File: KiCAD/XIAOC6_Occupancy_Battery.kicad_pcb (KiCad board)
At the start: 4 copper layers, 43.5 x 29.5 mm, 6 parts, among them U1 ZC362800_, U2 XIAO-ESP32-S3-SMD, U3 SHTC3

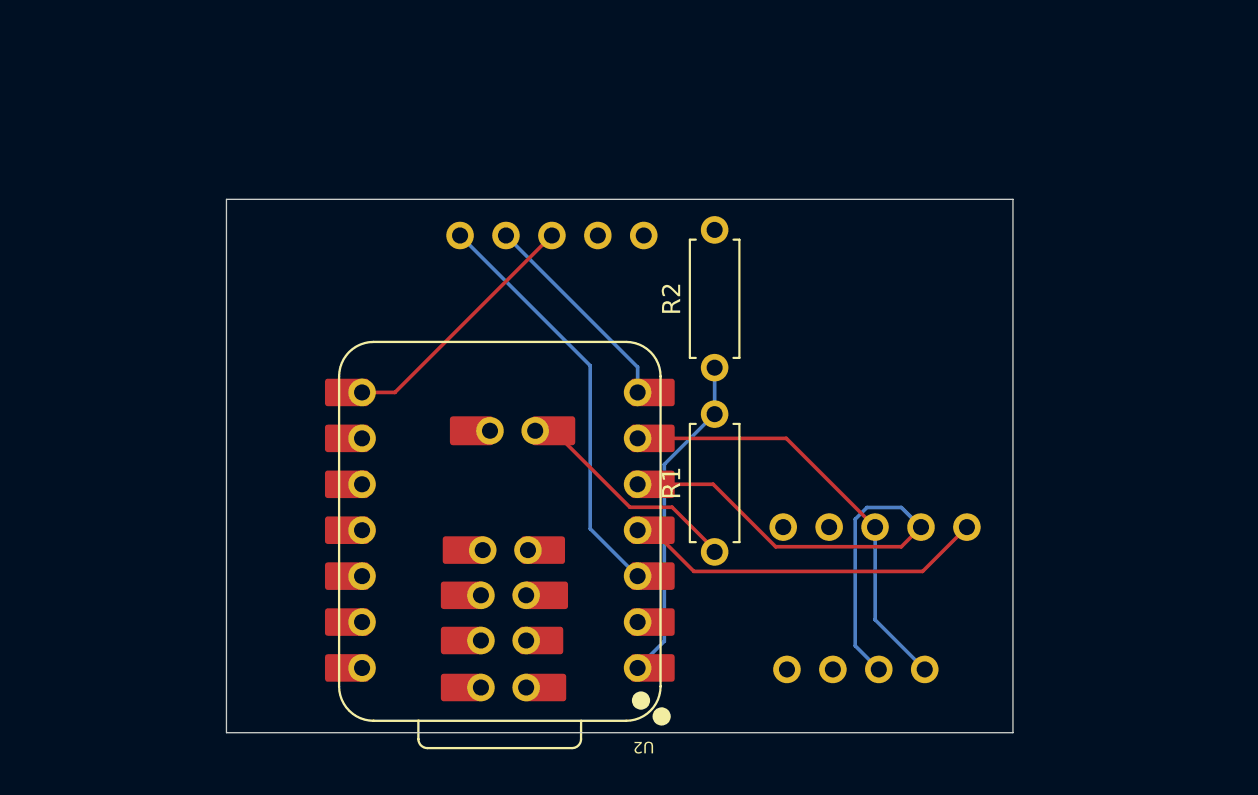
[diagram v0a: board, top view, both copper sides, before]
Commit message: update
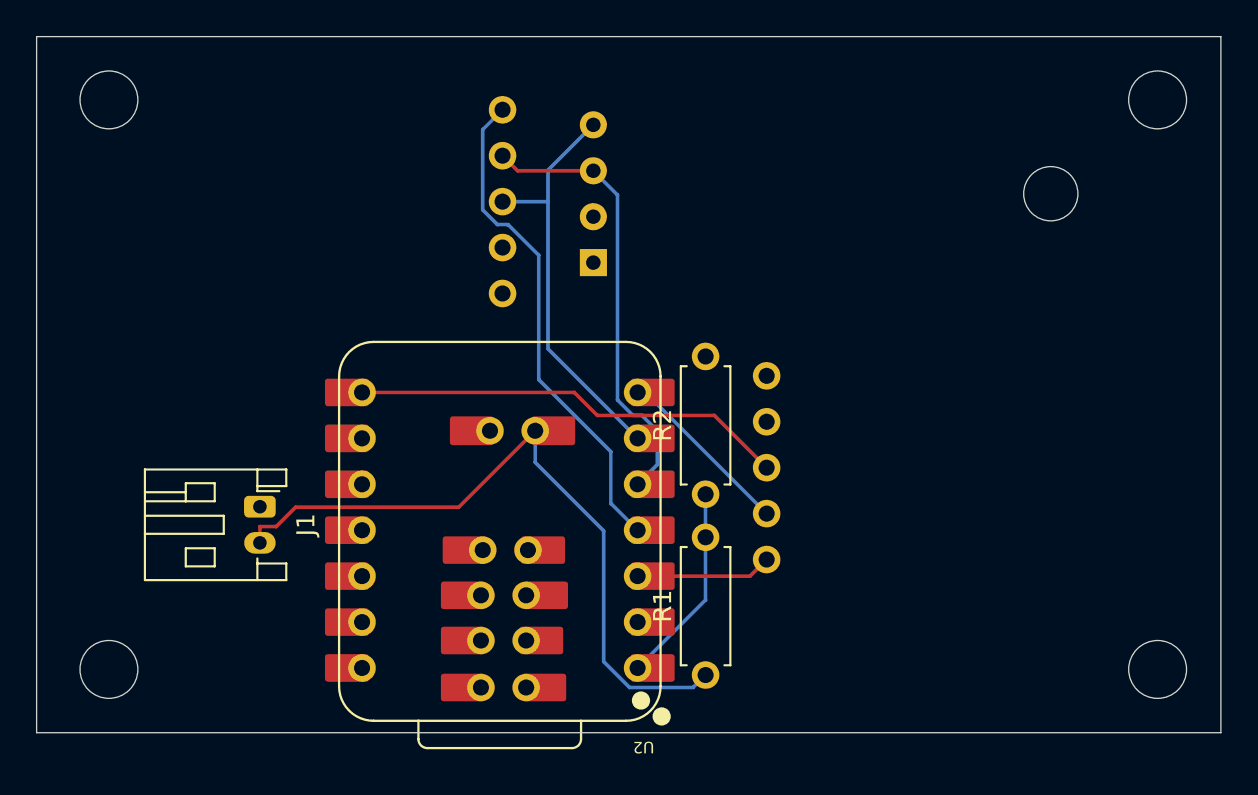
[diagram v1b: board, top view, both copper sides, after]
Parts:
- added H1: MountingHole_3.2mm_M3_DIN965, MountingHole:MountingHole_3.2mm_M3_DIN965, F.Cu at (145.5, 28.5)
- added H2: MountingHole_3.2mm_M3_DIN965, MountingHole:MountingHole_3.2mm_M3_DIN965, F.Cu at (145.5, 60.0)
- added H3: MountingHole_3.2mm_M3_DIN965, MountingHole:MountingHole_3.2mm_M3_DIN965, F.Cu at (87.5, 60.0)
- added H4: MountingHole_3.2mm_M3_DIN965, MountingHole:MountingHole_3.2mm_M3_DIN965, F.Cu at (87.5, 28.5)
- added J1: Conn_01x02_Socket, Connector_JST:JST_PH_S2B-PH-K_1x02_P2.00mm_Horizontal, F.Cu at (95.8, 51.0)
- U3: footprint Sensor:ASAIR_AM2302_P2.54mm_Vertical -> Sensor:ASAIR_AM2302_P2.54mm_Lead2.75mm_TabDown
- moved U1 27.5 mm to (108.0, 34.1), turned to 90 degrees
- moved U3 24.9 mm to (114.3, 37.5)
- moved U4 17.5 mm to (125.1, 48.8), turned to -90 degrees
- moved R2 7.02 mm to (120.5, 50.3)
- moved R1 6.83 mm to (120.5, 60.3)
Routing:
- net +BATT: track 12.8 -> 40.2 mm
- net LD2410S_EXT: track 23.7 -> 7.52 mm
- net RX: track 14.9 -> 24.9 mm
- net BH1750_ADDR: track 20.2 -> 28.4 mm
- net Net-(U2-GPIO0_A0_D0): track 19.2 -> 12.0 mm
- net SDA: track 30.8 -> 25.8 mm
- net TX: track 12.5 -> 10.7 mm
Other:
- board size 43.5 x 29.5 mm -> 65.5 x 38.5 mm
